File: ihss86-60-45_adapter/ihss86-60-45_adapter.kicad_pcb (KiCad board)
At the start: 2 copper layers, 90 x 40 mm, 17 parts, among them J2 T4140012081-000, J5 Conn_01x10_Socket, U1 MUN5233T1G, U2 MUN5233T1G, U3 MUN5233T1G, U4 MUN5233T1G

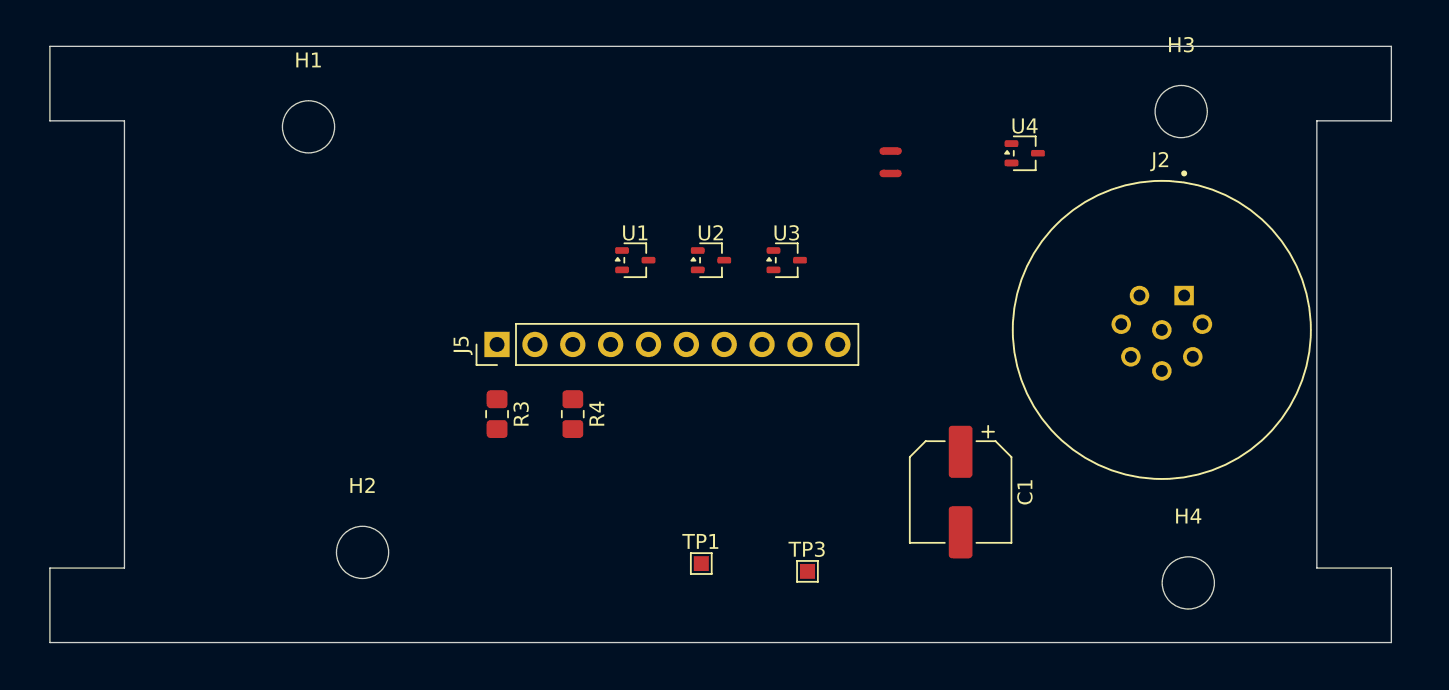
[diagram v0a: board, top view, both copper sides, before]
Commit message: Finished up basic PCB layout for the new servo adapter.
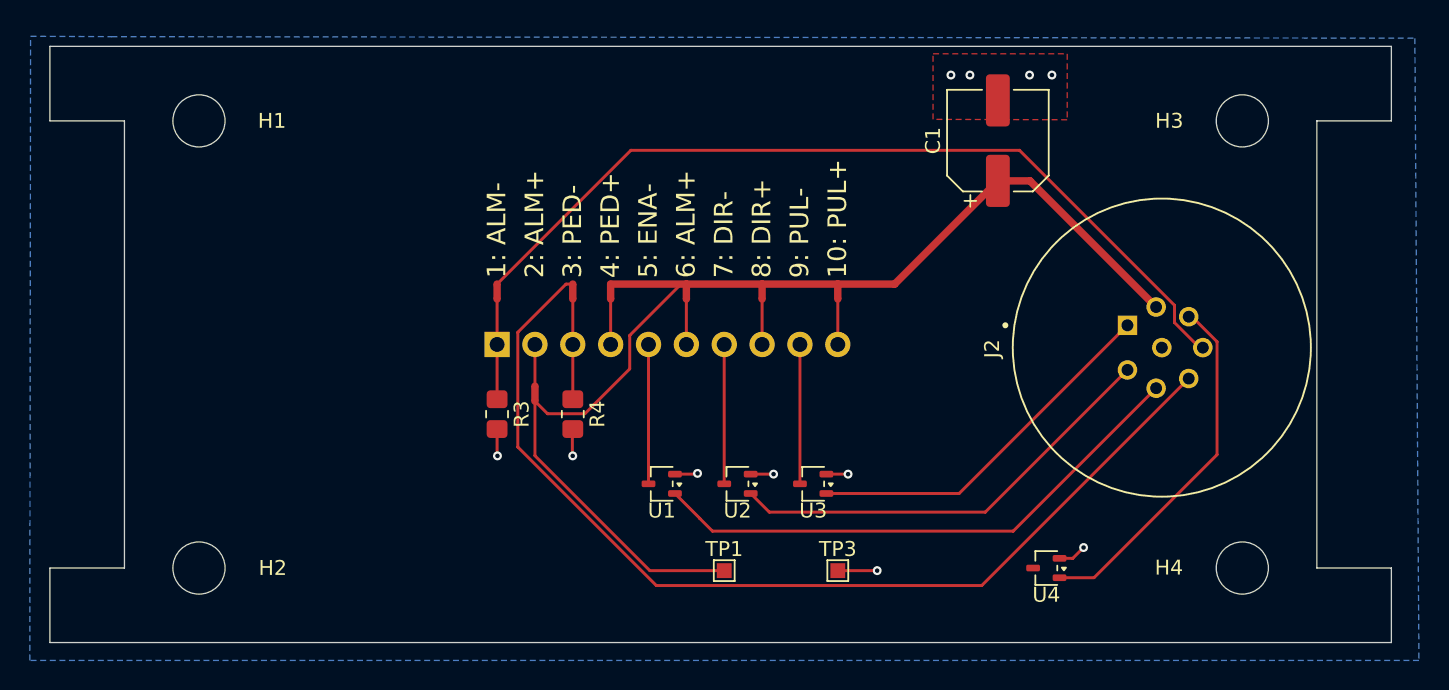
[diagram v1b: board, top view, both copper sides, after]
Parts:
- added NT2: NetTie_2, NetTie:NetTie-2_SMD_Pad0.5mm, F.Cu at (162.8, 91.5)
- added NT3: NetTie_2, NetTie:NetTie-2_SMD_Pad0.5mm, F.Cu at (167.9, 91.5)
- added NT4: NetTie_2, NetTie:NetTie-2_SMD_Pad0.5mm, F.Cu at (157.7, 91.5)
- added NT5: NetTie_2, NetTie:NetTie-2_SMD_Pad0.5mm, F.Cu at (152.6, 91.5)
- added NT6: NetTie_2, NetTie:NetTie-2_SMD_Pad0.5mm, F.Cu at (147.5, 98.3)
- J5: footprint Connector_PinHeader_2.54mm:PinHeader_1x10_P2.54mm_Vertical -> Connector_PinSocket_2.54mm:PinSocket_1x10_P2.54mm_Vertical; moved to B.Cu
- moved U4 27.9 mm to (181.8, 110.0), turned to 180 degrees
- moved NT7 27.6 mm to (145.0, 91.5), turned to -90 degrees
- moved C1 23.7 mm to (178.6, 81.3), turned to 90 degrees
- moved NT1 23.3 mm to (150.1, 91.5), turned to -90 degrees
- moved U1 15.1 mm to (156.0, 104.3), turned to 180 degrees
- moved U2 15.1 mm to (161.1, 104.3), turned to 180 degrees
- moved U3 15.1 mm to (166.2, 104.3), turned to 180 degrees
- moved H2 11.0 mm to (125.0, 110.0)
- moved H1 7.36 mm to (125.0, 80.0)
- moved H3 4.15 mm to (195.0, 80.0)
- moved H4 3.76 mm to (195.0, 110.0)
- moved TP3 2.04 mm to (167.9, 110.2)
- moved TP1 1.61 mm to (160.2, 110.2)
- moved J2 1.19 mm to (189.6, 95.2), turned to 90 degrees
- turned J5 to -90 degrees
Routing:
- net /+5V_Servo: track 0.00 -> 78.0 mm
- net /PED_OUT: track 0.00 -> 67.3 mm
- net /ALARM_OUT: track 0.00 -> 57.2 mm
- net /EN_IN: track 0.00 -> 37.3 mm
- net /DIR_IN: track 0.00 -> 29.7 mm
- net /STEP_IN: track 0.00 -> 24.9 mm
- net /AUX_IN: track 0.00 -> 24.6 mm
- net GND: track 0.00 -> 12.7 mm, vias 0 -> 11
- net /PUL-: track 0.00 -> 9.35 mm
- net /ENA-: track 0.00 -> 9.35 mm
- net /DIR-: track 0.00 -> 9.35 mm
- net /PED-: track 0.00 -> 6.72 mm
- net /ALM-: track 0.00 -> 6.72 mm
- net /PUL+: track 0.00 -> 3.05 mm
- net /PED+: track 0.00 -> 3.05 mm
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- added copper zone on B.Cu, net GND
- added copper zone on F.Cu, net GND
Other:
- board text added: "10: PUL+"
- board text added: "1: ALM-"
- board text added: "2: ALM+"
- board text added: "3: PED-"
- board text added: "4: PED+"
- board text added: "5: ENA-"
- board text added: "6: ALM+"
- board text added: "7: DIR-"
- board text added: "8: DIR+"
- board text added: "9: PUL-"
